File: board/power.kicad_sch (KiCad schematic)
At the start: 43 parts, among them Q1 BSS138, Q2 BSS138, Q3 BSS138, Q4 BSS138, Q5 BSS138, Q6 BSS138, Q7 BSS138, Q8 BSS138, Q9 BSS138, U1 OKI-78SR-5_1.5-W36H-C, U4 OKI-78SR-3.3_1.5-W36H-C

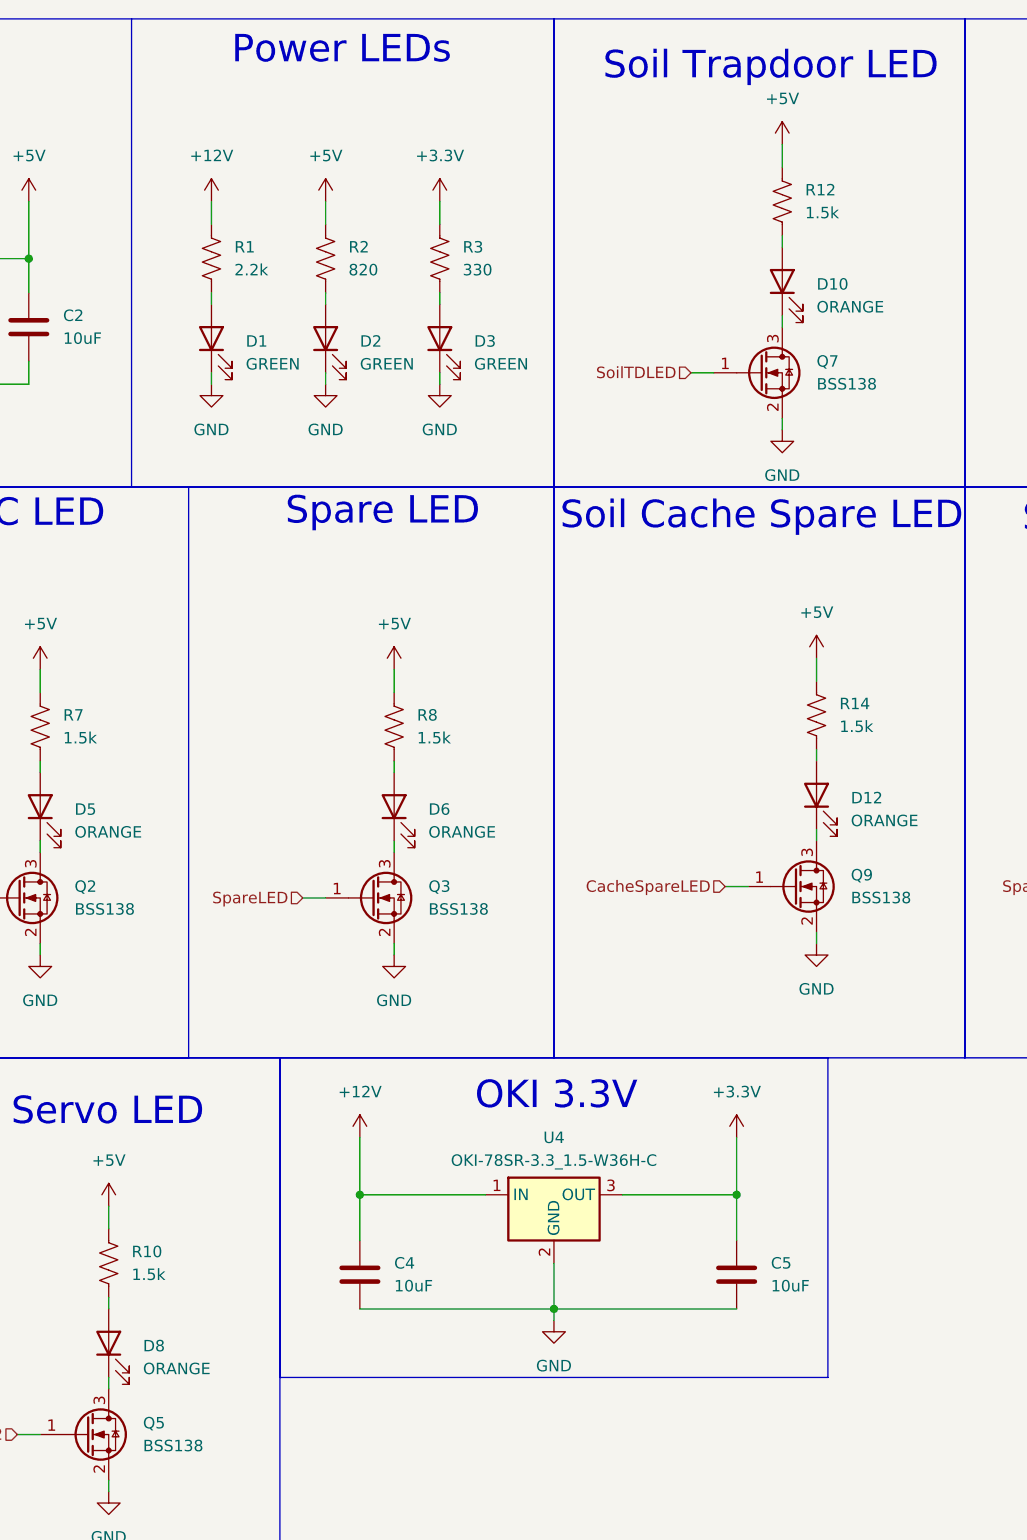
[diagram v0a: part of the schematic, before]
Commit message: Edited names and locations for readability
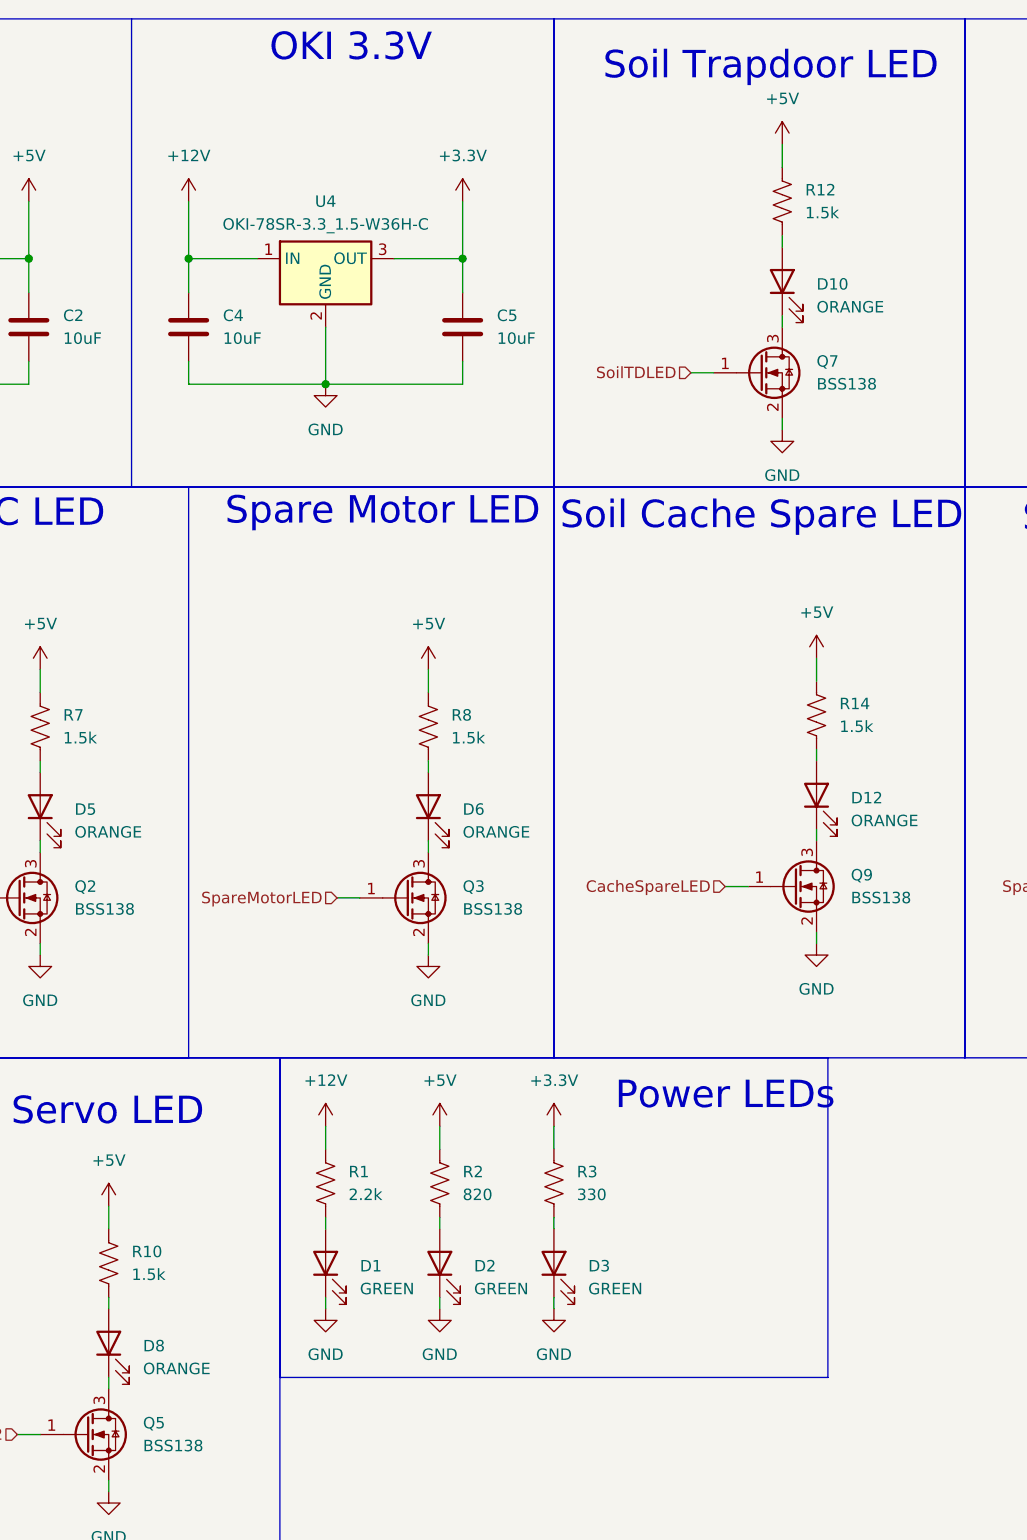
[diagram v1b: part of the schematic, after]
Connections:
- net SpareLED renamed SpareMotorLED
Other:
- note added: "Spare Motor LED"
- note removed: "Spare LED"
- moved on the sheet: C4, C5, D1, D2, D3, D6, Q3, R1, R2, R3, R8, U4
